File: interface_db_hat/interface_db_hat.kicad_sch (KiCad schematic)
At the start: 33 parts, among them J10 Conn_02x06_Counter_Clockwise, J2 DF19G-20P-1H52, J3 Conn_02x06_Counter_Clockwise, J6 Conn_01x04_Pin, J9 Conn_02x06_Counter_Clockwise

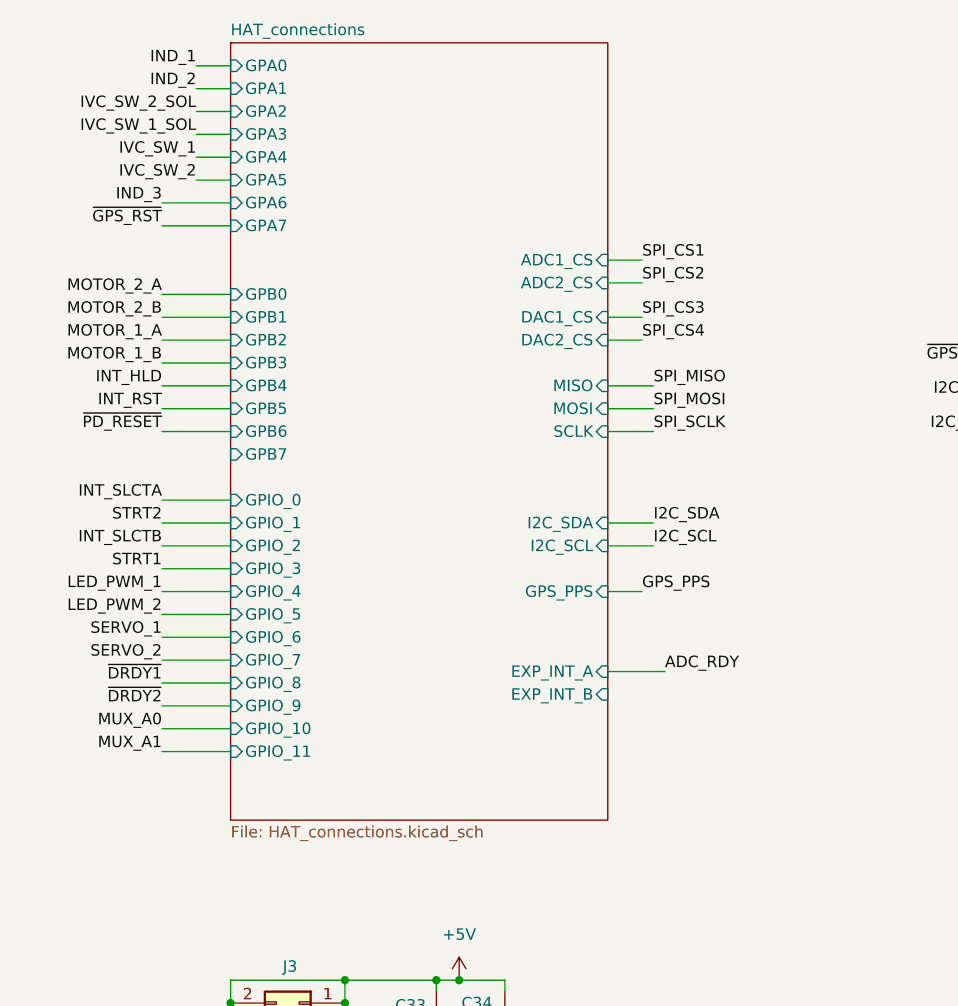
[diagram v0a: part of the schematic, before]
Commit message: fixed interface schematic
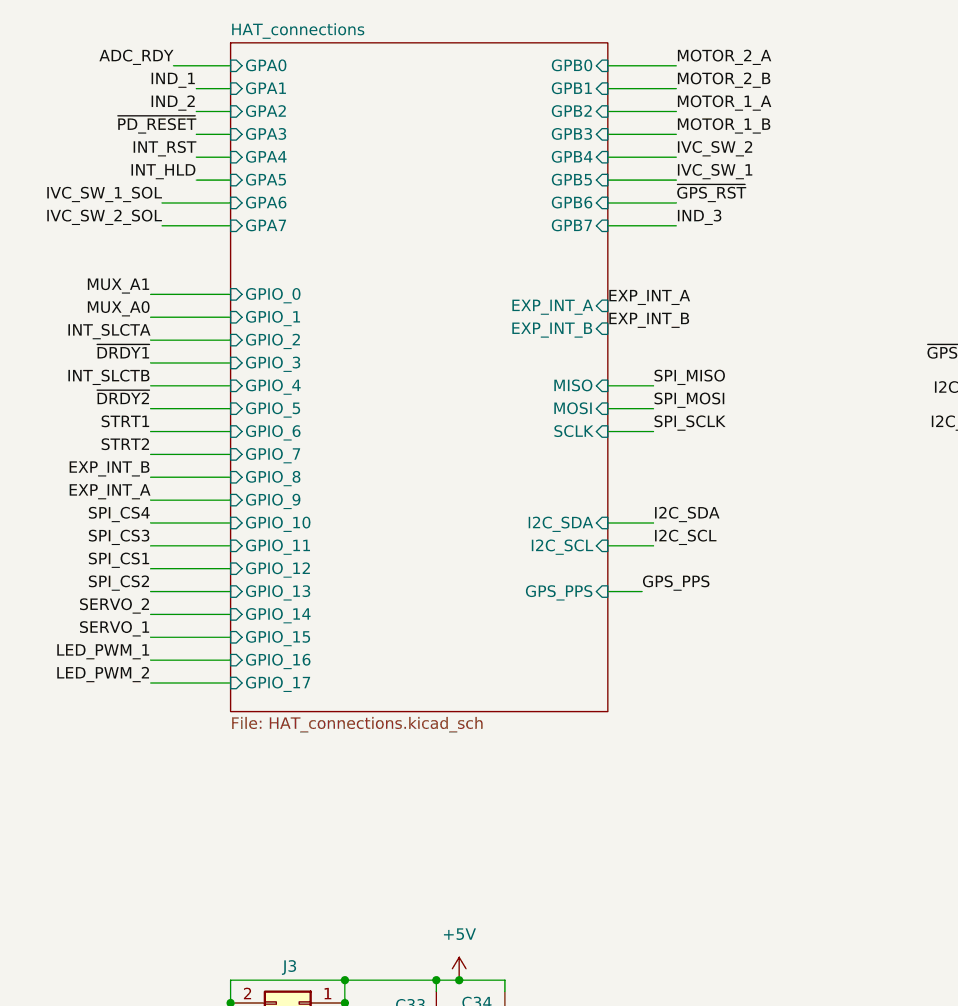
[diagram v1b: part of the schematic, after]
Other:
- sheet HAT_connections ports: added GPIO_12, GPIO_13, GPIO_14, GPIO_15, GPIO_16, GPIO_17; removed ADC1_CS, ADC2_CS, DAC1_CS, DAC2_CS
